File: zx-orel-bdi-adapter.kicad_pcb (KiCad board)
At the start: 2 copper layers, 100.3 x 80 mm, 22 parts, among them J1 Barrel_Jack_Switch, J2 DB9_Male, SW1 SW_Push_Dual, SW2 SW_DPDT_x2, U1 74LS30, U2 74LS27, U3 74LS04, U4 74LS640, U5 28C256

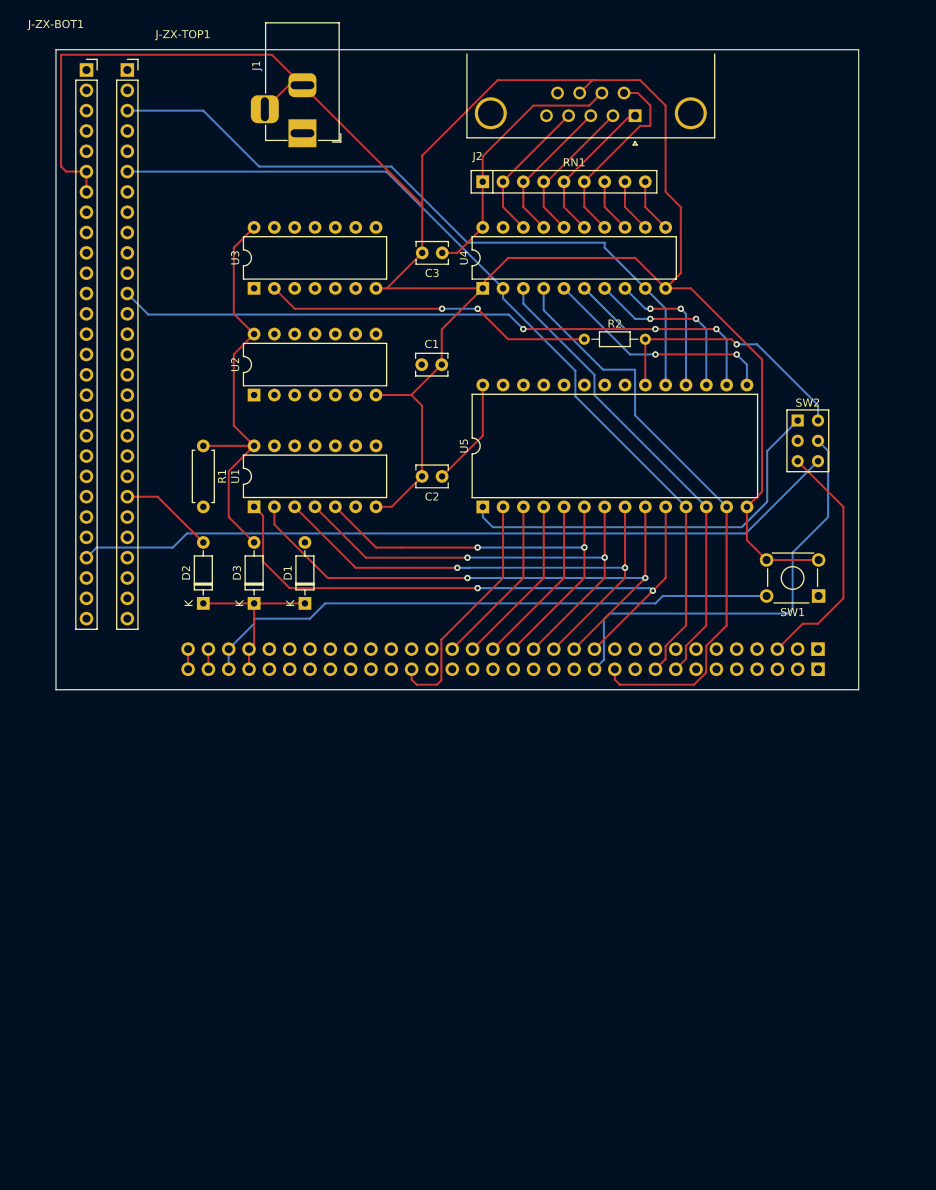
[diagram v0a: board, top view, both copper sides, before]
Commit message: finished orel bdi to zxbus design
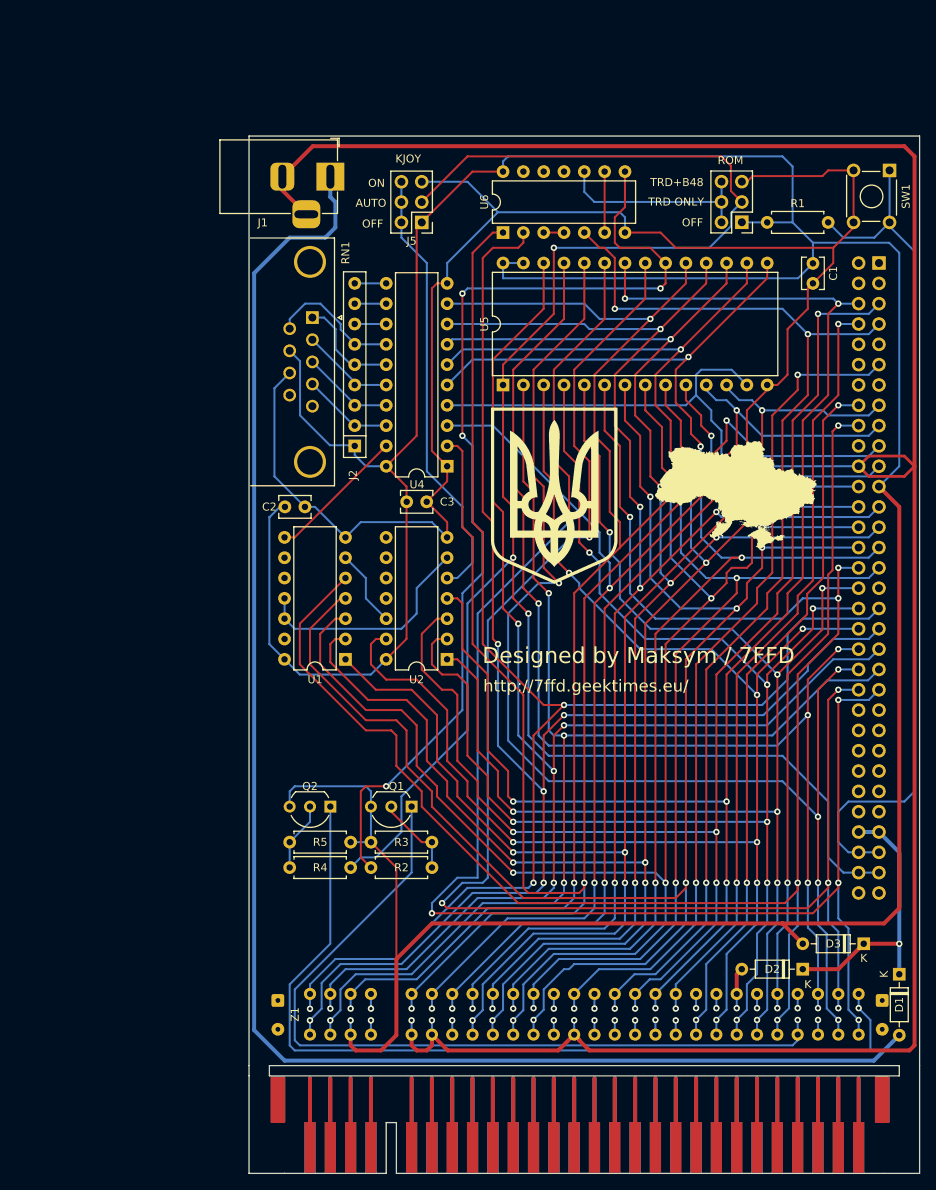
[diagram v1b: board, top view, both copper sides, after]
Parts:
- removed J-XA1, J-XB1: Conn_01x32_Female, Connector_PinSocket_2.54mm:PinSocket_1x32_P2.54mm_Vertical
- removed J-ZX-BOT1, J-ZX-TOP1: Conn_01x28_Female, Connector_PinSocket_2.54mm:PinSocket_1x28_P2.54mm_Vertical
- removed SW2: SW_DPDT_x2, Button_Switch_THT:SW_NKK_G1xJP
- removed U3: 74LS04, Package_DIP:DIP-14_W7.62mm
- added J3: Conn_02x32_Row_Letter_First, Connector_PinHeader_2.54mm:PinHeader_2x32_P2.54mm_Vertical, B.Cu at (141.0, 52.1)
- added J4: Conn_02x03_Odd_Even, Connector_PinHeader_2.54mm:PinHeader_2x03_P2.54mm_Vertical, F.Cu at (123.8, 47.0)
- added J5: Conn_02x03_Odd_Even, Connector_PinHeader_2.54mm:PinHeader_2x03_P2.54mm_Vertical, F.Cu at (83.8, 47.0)
- added MAP: UA CoA 16x22mm, Symbol:UA CoA 16x22mm Silk, F.Cu at (100.4, 64.6)
- added MAP: UA CoA 21x14mm, Symbol:UA map 21x14mm Silk, F.Cu at (123.8, 74.0)
- added Q1: BC558, Package_TO_SOT_THT:TO-92_Inline_Wide, F.Cu at (82.5, 120.0)
- added Q2: BC558, Package_TO_SOT_THT:TO-92_Inline_Wide, F.Cu at (72.4, 120.0)
- added R3: 680, Resistor_THT:R_Axial_DIN0207_L6.3mm_D2.5mm_P7.62mm_Horizontal, F.Cu at (85.1, 124.5)
- added R4: 2k2, Resistor_THT:R_Axial_DIN0207_L6.3mm_D2.5mm_P7.62mm_Horizontal, F.Cu at (74.9, 127.6)
- added R5: 680, Resistor_THT:R_Axial_DIN0207_L6.3mm_D2.5mm_P7.62mm_Horizontal, F.Cu at (67.3, 124.5)
- added REF**: SolderWire-0.1sqmm_1x02_P3.6mm_D0.4mm_OD1mm, Connector_Wire:SolderWire-0.1sqmm_1x02_P3.6mm_D0.4mm_OD1mm, B.Cu at (141.4, 144.2)
- added REF**: SolderWire-0.1sqmm_1x02_P3.6mm_D0.4mm_OD1mm, Connector_Wire:SolderWire-0.1sqmm_1x02_P3.6mm_D0.4mm_OD1mm, B.Cu at (65.8, 144.2)
- added U6: 74LS32, Package_DIP:DIP-14_W7.62mm, F.Cu at (94.0, 48.3)
- added Z1: ZXBUS, RobikBUS:ZXBUS Slot Connector, F.Cu at (67.9, 146.0)
- added ZXBUSEDGE: ZXBUS Edge Connector, RobikBUS:ZXBUS Edge Connector, B.Cu at (66.7, 162.7)
- R2: value 470 -> 2k2; footprint Resistor_THT:R_Axial_DIN0204_L3.6mm_D1.6mm_P7.62mm_Horizontal -> Resistor_THT:R_Axial_DIN0207_L6.3mm_D2.5mm_P7.62mm_Horizontal
- moved D2 87.8 mm to (131.4, 140.3), turned to 180 degrees
- moved D1 87.6 mm to (143.5, 141.0), turned to -90 degrees
- moved D3 87.3 mm to (139.1, 137.2), turned to 180 degrees
- moved R1 75.8 mm to (127.0, 47.0), turned to 0 degrees
- moved R2 71.2 mm to (77.5, 127.6)
- moved SW1 53.9 mm to (142.3, 40.5), turned to -90 degrees
- moved C1 50.5 mm to (132.7, 52.1), turned to -90 degrees
- moved J2 47.6 mm to (70.2, 58.9), turned to -90 degrees
- moved U2 40.9 mm to (87.0, 101.6), turned to 180 degrees
- moved RN1 36.7 mm to (75.4, 74.9), turned to 90 degrees
- moved C3 31.4 mm to (81.9, 81.9), turned to 0 degrees
- moved U4 22.7 mm to (87.0, 77.5), turned to 180 degrees
- moved U1 22.2 mm to (74.3, 101.6), turned to 180 degrees
- moved C2 20.0 mm to (66.7, 82.5), turned to 0 degrees
- moved U5 15.5 mm to (94.0, 67.3)
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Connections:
- R2 pad 1: Net-(R2-Pad1) -> Net-(U5-~{CS})
- R2 pad 2: //EXT_ROMCS -> Net-(Q1-B)
- U2 pad 10: /A14 -> unconnected-(U2-Pad10)
- U2 pad 11: //MREQ -> unconnected-(U2-Pad11)
- U2 pad 8: Net-(U2-Pad8) -> unconnected-(U2-Pad8)
- U2 pad 9: /A15 -> unconnected-(U2-Pad9)
- U5 pad 1: //BETA -> /TRDOS ROM ONLY
- U5 pad 20: //EXT_ROMCS -> Net-(U5-~{CS})
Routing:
- net (no net): track 0.00 -> 470.5 mm
- net +5V: track 153.7 -> 451.9 mm, vias 0 -> 1
- net /TRDOS ROM ONLY: track 0.00 -> 241.6 mm, vias 0 -> 3
- net GND: track 288.2 -> 503.5 mm, vias 0 -> 4
- net Net-(D1-A): track 0.00 -> 197.3 mm
- net /A11: track 0.00 -> 194.5 mm, vias 0 -> 5
- net /A10: track 0.00 -> 188.6 mm, vias 0 -> 5
- net /A14: track 0.00 -> 183.5 mm, vias 0 -> 5
- net /A15: track 0.00 -> 175.4 mm, vias 0 -> 3
- net /A13: track 0.00 -> 169.4 mm, vias 0 -> 5
- net //IORQ: track 0.00 -> 164.8 mm, vias 0 -> 5
- net /A07: track 21.5 -> 184.1 mm, vias 0 -> 7
- net /A09: track 0.00 -> 160.7 mm, vias 0 -> 5
- net /A04: track 54.7 -> 212.4 mm, vias 2 -> 5
- net //RD: track 30.4 -> 187.7 mm, vias 0 -> 6
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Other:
- board size 100.3 x 80 mm -> 83.8 x 129.7 mm
- board text added: "AUTO"
- board text added: "Designed by Maksym / 7FFD"
- board text added: "KJOY"
- board text added: "OFF"
- board text added: "ON"
- board text added: "ROM"
- board text added: "TRD ONLY"
- board text added: "TRD+B48"
- board text added: "http://7ffd.geektimes.eu/"
